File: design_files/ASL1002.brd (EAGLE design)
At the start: 11.7 x 5.5 mm, 5 parts

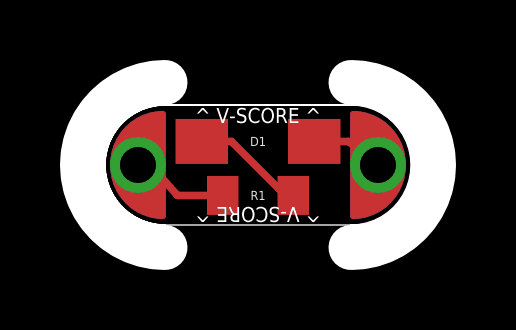
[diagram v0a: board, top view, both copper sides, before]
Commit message: update format
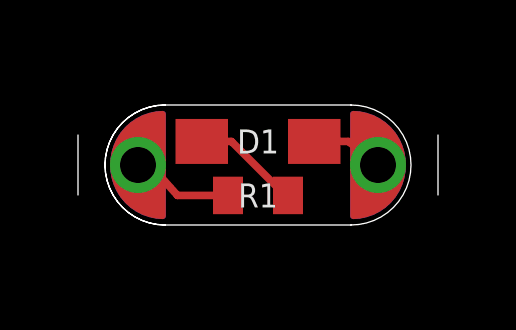
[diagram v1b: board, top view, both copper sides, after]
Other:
- board size 11.7 x 5.5 mm -> 12 x 4 mm
- board text removed: "^ V-SCORE ^"
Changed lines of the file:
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@@
 <setting verticaltext="up"/>
 </settings>
-<grid distance="1" unitdist="mm" unit="mm" style="lines" multiple="1" display="yes" altdistance="0.025" altunitdist="inch" altunit="inch"/>
+<grid distance="0.1" unitdist="mm" unit="mm" style="lines" multiple="1" display="yes" altdistance="0.025" altunitdist="inch" altunit="inch"/>
 <layers>
 <layer number="1" name="Top" color="4" fill="1" visible="yes" active="yes"/>
@@
 <layer number="54" name="bGND_GNDA" color="7" fill="1" visible="yes" active="yes"/>
 <layer number="56" name="wert" color="7" fill="1" visible="yes" active="yes"/>
+<layer number="57" name="tCAD" color="7" fill="1" visible="no" active="no"/>
+<layer number="58" name="bCAD" color="7" fill="1" visible="no" active="no"/>
+<layer number="59" name="Invisible" color="7" fill="1" visible="no" active="no"/>
+<layer number="61" name="stand" color="7" fill="1" visible="no" active="no"/>
+<layer number="88" name="SimResults" color="9" fill="1" visible="yes" active="yes"/>
+<layer number="89" name="SimProbes" color="9" fill="1" visible="yes" active="yes"/>
+<layer number="90" name="Modules" color="5" fill="1" visible="yes" active="yes"/>
 <layer number="91" name="Nets" color="2" fill="1" visible="no" active="no"/>
 <layer number="92" name="Busses" color="1" fill="1" visible="no" active="no"/>
@@
 <layer number="97" name="Info" color="7" fill="1" visible="no" active="no"/>
 <layer number="98" name="Guide" color="6" fill="1" visible="no" active="no"/>
+<layer number="99" name="SpiceOrder" color="5" fill="1" visible="no" active="no"/>
 <layer number="100" name="Muster" color="7" fill="1" visible="yes" active="yes"/>
 <layer number="101" name="Patch_Top" color="7" fill="1" visible="yes" active="yes"/>
@@
 <layer number="111" name="tGTest" color="4" fill="1" visible="no" active="no"/>
 <layer number="112" name="bGTest" color="1" fill="1" visible="no" active="no"/>
+<layer number="113" name="HENWAY_PKG" color="12" fill="1" visible="yes" active="yes"/>
+<layer number="114" name="50_Electronics_Plate" color="7" fill="1" visible="yes" active="yes"/>
+<layer number="115" name="henwayRES" color="5" fill="1" visible="yes" active="yes"/>
 <layer number="116" name="drillImage" color="7" fill="1" visible="yes" active="yes"/>
 <layer number="117" name="mPads" color="7" fill="1" visible="no" active="no"/>
@@
 <layer number="151" name="HeatSink" color="7" fill="1" visible="yes" active="yes"/>
 <layer number="152" name="mbDocu" color="7" fill="1" visible="no" active="no"/>
+<layer number="153" name="FabDoc1" color="6" fill="1" visible="no" active="no"/>
+<layer number="154" name="FabDoc2" color="2" fill="1" visible="no" active="no"/>
+<layer number="155" name="FabDoc3" color="7" fill="15" visible="no" active="no"/>
+<layer number="156" name="bCapacitor" color="7" fill="1" visible="yes" active="yes"/>
+<layer number="157" name="tResistor" color="7" fill="1" visible="yes" active="yes"/>
+<layer number="158" name="bResistor" color="7" fill="1" visible="yes" active="yes"/>
+<layer number="159" name="henwayCAP" color="13" fill="1" visible="yes" active="yes"/>
 <layer number="191" name="mNets" color="7" fill="1" visible="no" active="no"/>
 <layer number="192" name="mBusses" color="7" fill="1" visible="no" active="no"/>
@@
 <layer number="223" name="223bmp" color="7" fill="1" visible="yes" active="yes"/>
 <layer number="224" name="224bmp" color="7" fill="1" visible="yes" active="yes"/>
+<layer number="231" name="Eagle3D_PG1" color="7" fill="1" visible="yes" active="yes"/>
+<layer number="232" name="Eagle3D_PG2" color="7" fill="1" visible="yes" active="yes"/>
+<layer number="233" name="Eagle3D_PG3" color="7" fill="1" visible="yes" active="yes"/>
 <layer number="248" name="Housing" color="7" fill="1" visible="yes" active="yes"/>
 <layer number="249" name="Edge" color="7" fill="1" visible="yes" active="yes"/>
@@
 <wire x1="69.85" y1="50.8" x2="0" y2="50.8" width="0.127" layer="48"/>
 <wire x1="0" y1="50.8" x2="0" y2="0" width="0.127" layer="48"/>
-<dimension x1="25.1" y1="20" x2="14.9" y2="20" x3="20" y3="24.524653125" layer="48"/>
+<dimension x1="25.1" y1="22" x2="14.9" y2="22" x3="20" y3="26.524653125" layer="48"/>
 <text x="48.111025" y="4.365003125" size="0.889" layer="48">TinyLily LED - 1206</text>
 <text x="44.986825" y="1.7714" size="0.889" layer="48">AS-PCB-ASL1002</text>
@@
 <text x="16.718715625" y="19.35918125" size="1.5" layer="22" rot="MR90">-</text>
 <text x="22.6168625" y="19.145540625" size="1.5" layer="22" rot="MR0">+</text>
-<dimension x1="17" y1="22" x2="17" y2="18" x3="8.83319375" y3="20" layer="48"/>
+<dimension x1="14.9" y1="22" x2="14.9" y2="18" x3="6.73319375" y3="20" layer="48"/>
 <text x="40.4876" y="15.040596875" size="0.4572" layer="48" ratio="10">Released under the Creative Commons Attribution Share-Alike 3.0 License</text>
 <text x="40.4876" y="14.278596875" size="0.4572" layer="48" ratio="10">http://creativecommons.org/licenses/by-sa/3.0</text>
 <text x="40.4876" y="13.008596875" size="0.4572" layer="48" ratio="10">Original Arduino Uno Design by Team Arduino</text>
 <text x="40.513" y="11.687796875" size="0.4572" layer="48" ratio="10">TinyDuino, TinyLily and TinyShield Designs by TinyCircuits</text>
-<wire x1="16.9" y1="17.25" x2="16.9" y2="22.75" width="1.5" layer="46" curve="-180"/>
 <wire x1="23.1" y1="18" x2="23.1" y2="22" width="0.0254" layer="20" curve="180"/>
 <wire x1="16.9" y1="22" x2="16.9" y2="18" width="0.0254" layer="20" curve="180"/>
 <wire x1="23.1" y1="22" x2="16.9" y2="22" width="0.0254" layer="20"/>
 <wire x1="16.9" y1="18" x2="23.1" y2="18" width="0.0254" layer="20"/>
-<wire x1="23.1" y1="18" x2="23.1" y2="22" width="0.0254" layer="108" curve="180"/>
 <wire x1="16.9" y1="22" x2="16.9" y2="18" width="0.0254" layer="20" curve="180"/>
-<wire x1="23.1" y1="22" x2="16.9" y2="22" width="0.0254" layer="108"/>
 <text x="40.513" y="12.373596875" size="0.4572" layer="48" ratio="10">LilyPad Arduino Design by Leah Buechley and Sparkfun Electronics</text>
-<wire x1="23.1" y1="22.75" x2="23.1" y2="17.25" width="1.5" layer="46" curve="-180"/>
-<wire x1="14.9" y1="18" x2="16.9" y2="18" width="0.0254" layer="20"/>
-<wire x1="23.1" y1="18" x2="25.1" y2="18" width="0.0254" layer="20"/>
-<wire x1="25.1" y1="22" x2="14.9" y2="22" width="0.0254" layer="20"/>
-<text x="20" y="21.4" size="0.5" layer="20" align="bottom-center">^ V-SCORE ^</text>
-<text x="20" y="18.6" size="0.5" layer="20" rot="SR180" align="bottom-center">^ V-SCORE ^</text>
+<wire x1="14" y1="21" x2="14" y2="19" width="0.0254" layer="20"/>
+<wire x1="26" y1="21" x2="26" y2="19" width="0.0254" layer="20"/>
 </plain>
 <attributes>
@@
 <contactref element="D1" pad="2"/>
 <contactref element="R1" pad="1"/>
-<wire x1="21.175" y1="18.9858" x2="21.125" y2="19.1858" width="0.254" layer="1"/>
+<wire x1="21" y1="18.9858" x2="21.125" y2="19.1858" width="0.254" layer="1"/>
 <wire x1="21.125" y1="19.1858" x2="20.7" y2="19.2" width="0.254" layer="1"/>
 <wire x1="20.7" y1="19.2" x2="19.115" y2="20.785" width="0.254" layer="1"/>
@@
 <contactref element="U$1" pad="1"/>
 <contactref element="R1" pad="2"/>
-<wire x1="18.825" y1="18.9858" x2="17.3142" y2="18.9858" width="0.254" layer="1"/>
+<wire x1="19" y1="18.9858" x2="17.3142" y2="18.9858" width="0.254" layer="1"/>
 <wire x1="17.3142" y1="18.9858" x2="16.5" y2="19.9" width="0.254" layer="1"/>
 <wire x1="16.5" y1="19.9" x2="16.1" y2="19.9" width="0.254" layer="1"/>
